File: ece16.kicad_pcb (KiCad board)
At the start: 2 copper layers, 50 x 36 mm, 60 parts, among them U1 LP5907MFX-3.3, U2 ESP32-S3-MINI-1-N8, U3 ADXL335, U4 DM-OLED096-636, U5 LP5907MFX-1.8, U6 MAX30101EFD_T

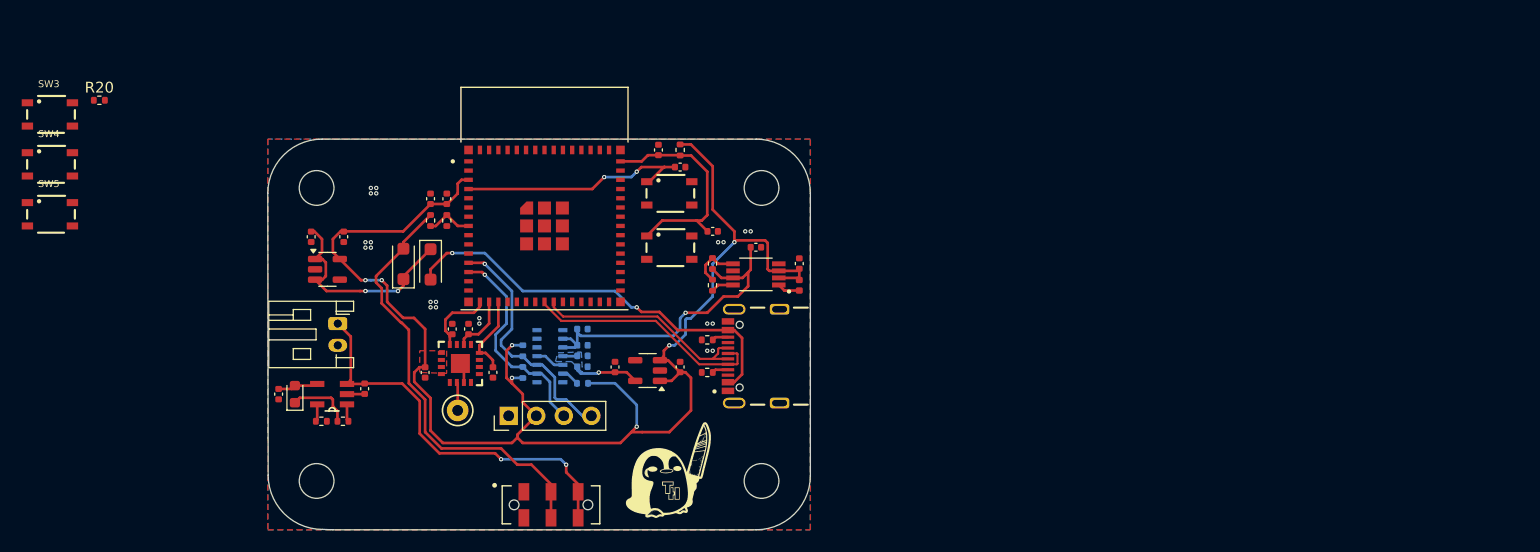
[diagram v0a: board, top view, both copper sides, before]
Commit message: Before you delete and reset everything
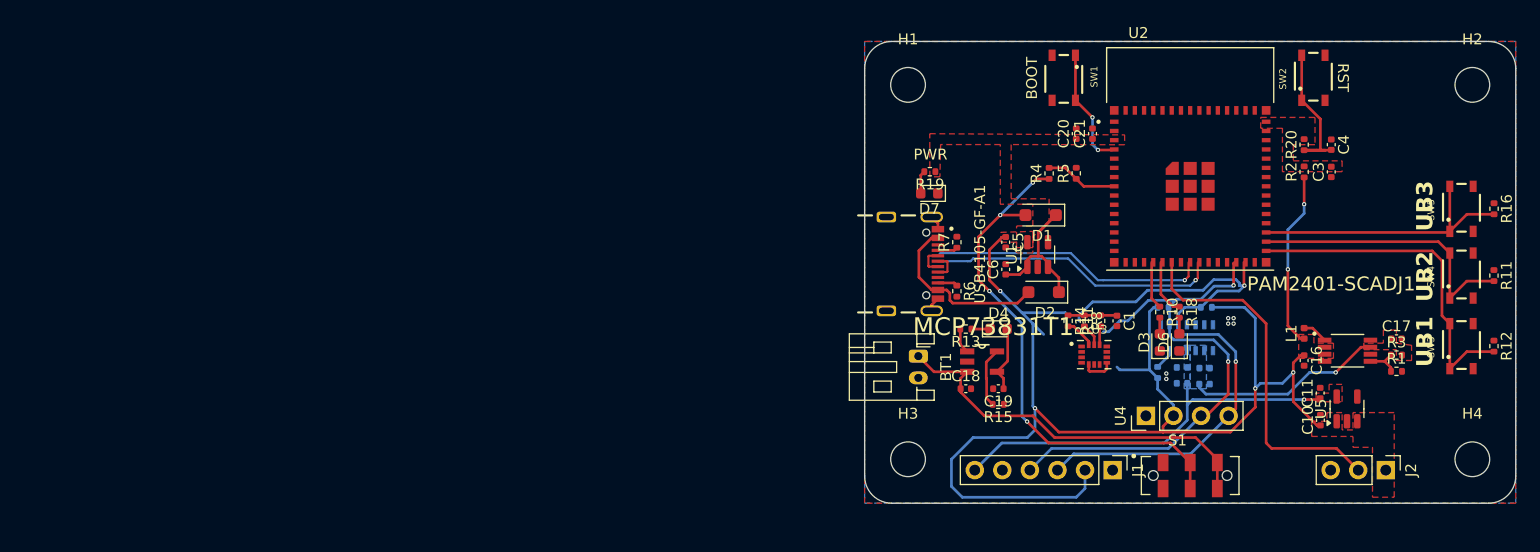
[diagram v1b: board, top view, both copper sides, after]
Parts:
- removed C2, C7, C8, C9: 0.1uF, Capacitor_SMD:C_0402_1005Metric
- removed G***: LOGO, LOGO
- removed the R14 at (133.5, 58.5)
- removed the R8 at (133.5, 60.5)
- removed TP1: TestPoint, TestPoint:TestPoint_Keystone_5000-5004_Miniature
- added D3: LED, LED_SMD:LED_0603_1608Metric, F.Cu at (192.2, 57.7)
- added D6: LED, LED_SMD:LED_0603_1608Metric, F.Cu at (194.0, 57.7)
- added D7: LED, LED_SMD:LED_0603_1608Metric, F.Cu at (171.0, 44.0)
- added J1: Conn_01x06_Socket, Connector_PinHeader_2.54mm:PinHeader_1x06_P2.54mm_Vertical, F.Cu at (187.8, 69.5)
- added J2: Conn_01x03_Pin, Connector_PinHeader_2.54mm:PinHeader_1x03_P2.54mm_Vertical, F.Cu at (213.0, 69.5)
- added R10: 510, Resistor_SMD:R_0402_1005Metric, F.Cu at (192.2, 54.9)
- added R11: 1k, Resistor_SMD:R_0402_1005Metric, F.Cu at (223.0, 51.6)
- added R11: 1k, Resistor_SMD:R_0402_1005Metric, F.Cu at (186.8, 55.8)
- added R12: 1k, Resistor_SMD:R_0402_1005Metric, F.Cu at (223.0, 58.1)
- added R14: 1k, Resistor_SMD:R_0402_1005Metric, F.Cu at (183.8, 55.8)
- added R14: 1k, Resistor_SMD:R_0402_1005Metric, B.Cu at (196.5, 54.5)
- added R16: 1k, Resistor_SMD:R_0402_1005Metric, F.Cu at (223.0, 45.4)
- added R18: 510, Resistor_SMD:R_0402_1005Metric, F.Cu at (194.0, 54.9)
- added R19: 510, Resistor_SMD:R_0402_1005Metric, F.Cu at (171.0, 42.0)
- added R8: 1k, Resistor_SMD:R_0402_1005Metric, F.Cu at (185.2, 55.8)
- added R8: 1k, Resistor_SMD:R_0402_1005Metric, B.Cu at (192.5, 54.5)
- U3: value ADXL335 -> LSM6DSOXTR; footprint ADXL335:LFCSP-16 -> LSM6DSOXTR:PQFN50P250X300X86-14N
- moved SW3 131.8 mm to (220.0, 58.1), turned to 90 degrees
- moved SW4 130.5 mm to (220.0, 51.6), turned to 90 degrees
- moved SW5 130.1 mm to (220.0, 45.4), turned to 90 degrees
- moved R20 111.1 mm to (205.5, 39.5), turned to 90 degrees
- moved H2 75.0 mm to (221.0, 34.0)
- moved H4 70.1 mm to (221.0, 68.5)
- moved C19 66.3 mm to (177.3, 62.0), turned to 180 degrees
- moved U1 65.5 mm to (180.9, 49.6), turned to 90 degrees
- moved D4 65.1 mm to (177.3, 56.5), turned to 0 degrees
- moved C11 65.0 mm to (207.0, 62.4)
- moved U5 64.5 mm to (209.4, 63.9), turned to 90 degrees
- moved C6 64.1 mm to (178.0, 51.0), turned to 90 degrees
- moved R3 63.6 mm to (214.0, 58.9), turned to 0 degrees
- moved R1 63.5 mm to (214.0, 60.4), turned to 0 degrees
- moved R15 62.4 mm to (177.3, 63.4)
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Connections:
- net /STAT renamed Net-(MCP73831T1-STAT)
- C1 pad 1: /Ay -> +3V3
- C19 pad 1: Net-(D4-A) -> +5V
- D4 pad 2: Net-(D4-A) -> +5V
- MCP73831T1 pad 4: Net-(D4-A) -> +5V
- U2 pad 12: /SDA -> unconnected-(U2-IO8-Pad12)
- U2 pad 13: /SCL -> unconnected-(U2-IO9-Pad13)
- U2 pad 19: unconnected-(U2-IO15-Pad19) -> /U-LED1
- U2 pad 20: unconnected-(U2-IO16-Pad20) -> /U-LED2
- U2 pad 21: unconnected-(U2-IO17-Pad21) -> /T1
- U2 pad 28: unconnected-(U2-IO33-Pad28) -> /SCL
- U2 pad 29: unconnected-(U2-IO34-Pad29) -> /SDA
- U2 pad 31: unconnected-(U2-IO35-Pad31) -> /UB1
- U2 pad 32: unconnected-(U2-IO36-Pad32) -> /UB2
- U2 pad 33: unconnected-(U2-IO37-Pad33) -> /UB3
- U3 pad 1: unconnected-(U3-NC-Pad1) -> GND
- U3 pad 10: /Ay -> unconnected-(U3-OCS_AUX-Pad10)
- U3 pad 12: /Ax -> Net-(U3-CS)
- U3 pad 13: unconnected-(U3-NC-Pad13) -> /SCL
- U3 pad 14: +3V3 -> /SDA
- U3 pad 2: Net-(U3-ST) -> GND
- U3 pad 4: unconnected-(U3-NC-Pad4) -> /INT1
- U3 pad 5: GND -> +3V3
- U3 pad 8: /Az -> +3V3
- U3 pad 9: unconnected-(U3-NC-Pad9) -> /INT2
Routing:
- net /SDA: track 22.6 -> 61.5 mm, vias 1 -> 2
- net /T1: track 0.00 -> 33.0 mm
- net /SCL: track 19.7 -> 52.5 mm, vias 1 -> 2
- net /UB1: track 0.00 -> 31.5 mm
- net +1.8V: track 7.51 -> 37.4 mm
- net /UB2: track 0.00 -> 26.2 mm
- net /UB3: track 0.00 -> 26.0 mm
- net /EN: track 20.7 -> 0.00 mm
- net +5V: track 38.5 -> 22.8 mm, vias 2 -> 0
- net Net-(C4-Pad2): track 0.00 -> 13.9 mm
- net /VLED: track 30.7 -> 18.1 mm
- net /Boot: track 22.1 -> 11.1 mm
- net /DP: track 20.6 -> 29.5 mm, vias 0 -> 1
- net +BATT: track 40.0 -> 48.9 mm, vias 0 -> 4
- net /Az: track 7.60 -> 0.00 mm
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- added copper zone on F.Cu, net +1.8V
- added copper zone on F.Cu, net /EN
- added copper zone on B.Cu, net /VLED
- added copper zone on F.Cu, net /VLED
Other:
- board size 50 x 36 mm -> 60 x 42.5 mm
- board text added: "BOOT"
- board text added: "PWR"
- board text added: "RST"
- board text added: "UB1"
- board text added: "UB2"
- board text added: "UB3"
